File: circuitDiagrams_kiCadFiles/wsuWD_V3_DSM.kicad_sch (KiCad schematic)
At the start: 33 parts, among them J2 Screw Terminal, U1 MCP2561-E-P, U2 LD1086DT50TR, U3 ATmega644A-P, U4 FT232RL_BOB, U7 MAX7219, U8 MCP2515-xSO, X1 ACO-20MHz-A

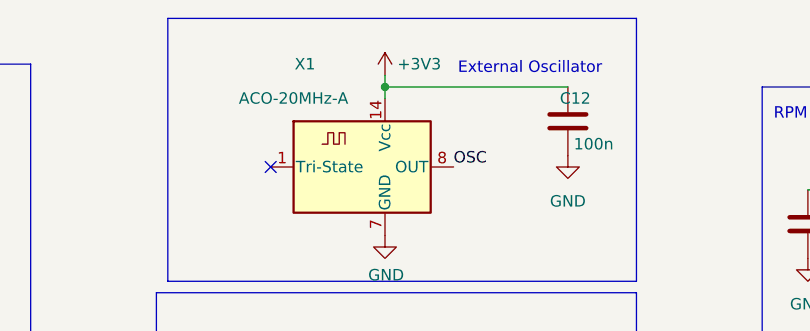
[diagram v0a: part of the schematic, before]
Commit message: Included new datasheets
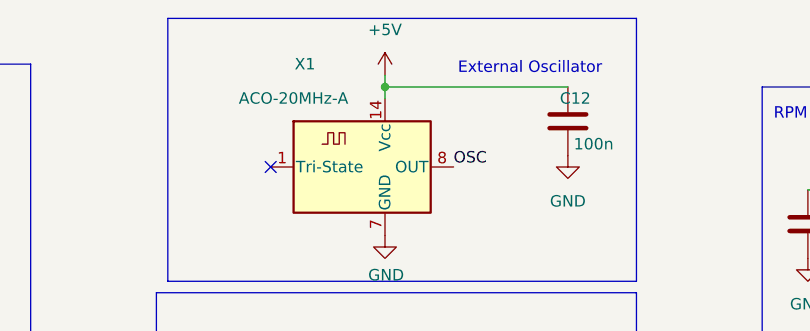
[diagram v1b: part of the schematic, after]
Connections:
- net +3V3: no longer C12.2, X1.14 (Vcc)
- net +5V: now also C12.2, X1.14 (Vcc)
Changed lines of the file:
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@@
     (pin "2")
-  )
-  (symbol (lib_id "power:+3V3") (at 161.29 20.32 0) (unit 1)
-    (in_bom yes) (on_board yes)
-    (property "Reference" "#PWR0119" (id 0) (at 161.29 24.13 0)
-      (effects (font (size 1.27 1.27)) hide)
-    )
-    (property "Value" "+3V3" (id 1) (at 165.1 19.05 0))
-    (property "Footprint" "" (id 2) (at 161.29 20.32 0)
-      (effects (font (size 1.27 1.27)) hide)
-    )
-    (property "Datasheet" "" (id 3) (at 161.29 20.32 0)
-      (effects (font (size 1.27 1.27)) hide)
-    )
-    (pin "1")
   )
   (symbol (lib_id "Device:C") (at 104.14 25.4 0) (unit 1)
@@
     (pin "1")
     (pin "2")
+  )
+  (symbol (lib_id "power:+5V") (at 161.29 20.32 0) (unit 1)
+    (in_bom yes) (on_board yes) (fields_autoplaced)
+    (property "Reference" "#PWR?" (id 0) (at 161.29 24.13 0)
+      (effects (font (size 1.27 1.27)) hide)
+    )
+    (property "Value" "+5V" (id 1) (at 161.29 15.24 0))
+    (property "Footprint" "" (id 2) (at 161.29 20.32 0)
+      (effects (font (size 1.27 1.27)) hide)
+    )
+    (property "Datasheet" "" (id 3) (at 161.29 20.32 0)
+      (effects (font (size 1.27 1.27)) hide)
+    )
+    (pin "1")
   )
   (symbol (lib_id "Device:LED") (at 257.81 100.33 90) (unit 1)
@@
       (reference "#PWR0118") (unit 1) (value "GND") (footprint "")
     )
-    (path "/00000000-0000-0000-0000-0000601b9c3a"
-      (reference "#PWR0119") (unit 1) (value "+3V3") (footprint "")
-    )
     (path "/00000000-0000-0000-0000-0000601a7b42"
       (reference "#PWR0120") (unit 1) (value "GND") (footprint "")
@@
       (reference "#PWR0135") (unit 1) (value "+5V") (footprint "")
     )
+    (path "/29580cbd-a1ab-4026-982c-7d252173a460"
+      (reference "#PWR?") (unit 1) (value "+5V") (footprint "")
+    )
     (path "/00000000-0000-0000-0000-000060146acc"
